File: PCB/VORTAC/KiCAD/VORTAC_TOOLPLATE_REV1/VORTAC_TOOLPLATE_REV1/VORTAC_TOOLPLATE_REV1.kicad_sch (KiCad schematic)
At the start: 6 parts, among them J1 Conn_01x07, J2 Conn_01x02

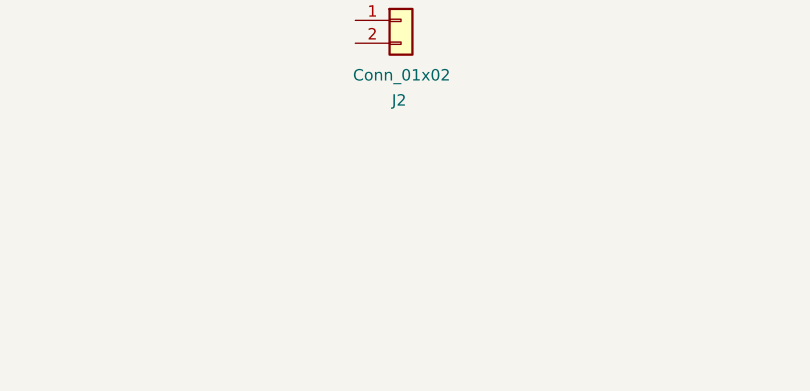
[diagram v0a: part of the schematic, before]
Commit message: MEIN BEEEEEIIIINNNN
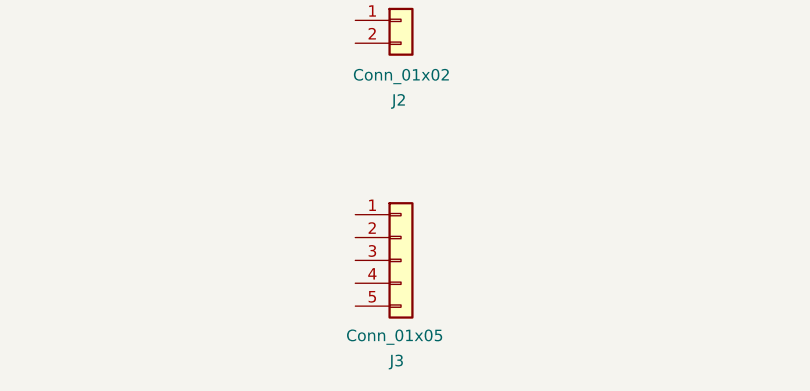
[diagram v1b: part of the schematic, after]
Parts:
- added J3: Conn_01x05, Vortac:Toolplate_Solderpoint_01x05_Data, symbol Connector_Generic:Conn_01x05
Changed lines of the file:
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@@
+	)
+	(symbol
+		(lib_id "Connector_Generic:Conn_01x05")
+		(at 71.12 106.68 0)
+		(unit 1)
+		(exclude_from_sim no)
+		(in_bom yes)
+		(on_board yes)
+		(dnp no)
+		(property "Reference" "J3"
+			(at 69.85 117.856 0)
+			(effects
+				(font
+					(size 1.27 1.27)
+				)
+				(justify left)
+			)
+		)
+		(property "Value" "Conn_01x05"
+			(at 65.024 115.062 0)
+			(effects
+				(font
+					(size 1.27 1.27)
+				)
+				(justify left)
+			)
+		)
+		(property "Footprint" "Vortac:Toolplate_Solderpoint_01x05_Data"
+			(at 71.12 118.618 0)
+			(effects
+				(font
+					(size 1.27 1.27)
+				)
+				(hide yes)
+			)
+		)
+		(property "Datasheet" "~"
+			(at 71.12 106.68 0)
+			(effects
+				(font
+					(size 1.27 1.27)
+				)
+				(hide yes)
+			)
+		)
+		(property "Description" "Generic connector, single row, 01x05, script generated (kicad-library-utils/schlib/autogen/connector/)"
+			(at 71.12 106.68 0)
+			(effects
+				(font
+					(size 1.27 1.27)
+				)
+				(hide yes)
+			)
+		)
+		(pin "4"
+		)
+		(pin "3"
+		)
+		(pin "1"
+		)
+		(pin "2"
+		)
+		(pin "5"
+		)
+		(instances
+			(project ""
+				(path "/b23b3086-82ed-4285-9d49-d03b4e41a1a0"
+					(reference "J3")
+					(unit 1)
+				)
+			)
+		)
 	)
 	(symbol
